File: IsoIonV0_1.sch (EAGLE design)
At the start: 52 parts, among them IC1 MCP3221, IC2 MCP4017-100K, IC4 TL072, IC5 TPS60400DBV

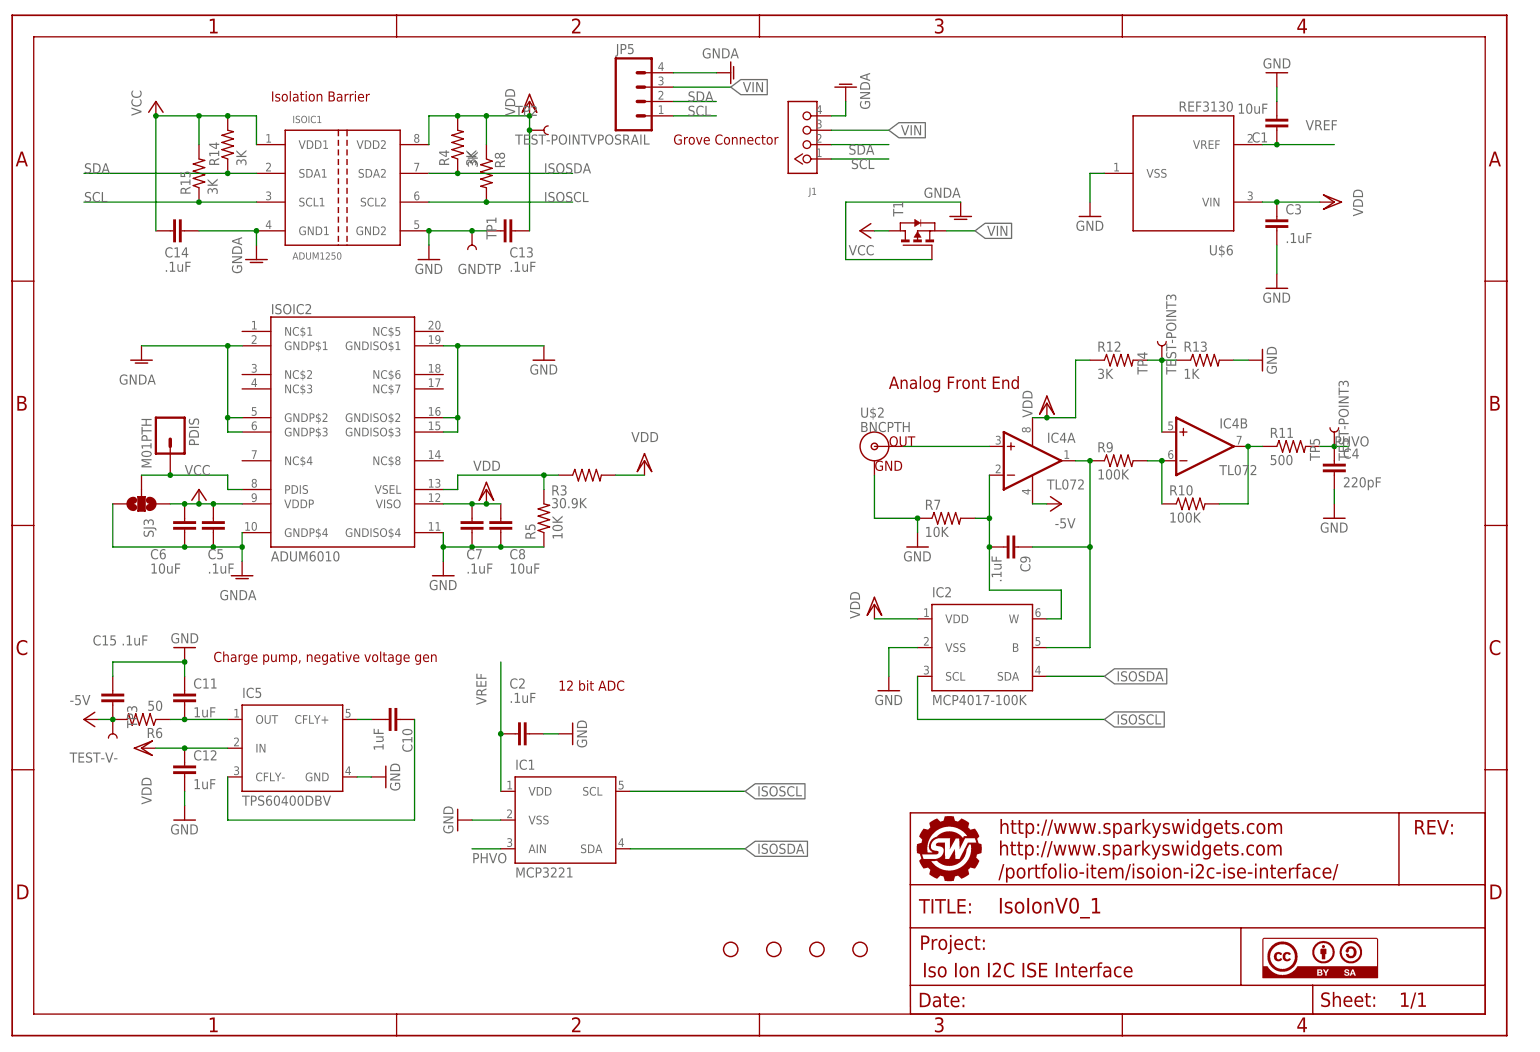
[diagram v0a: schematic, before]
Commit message: Cleaned up sch small silkscreen adjustment on brd
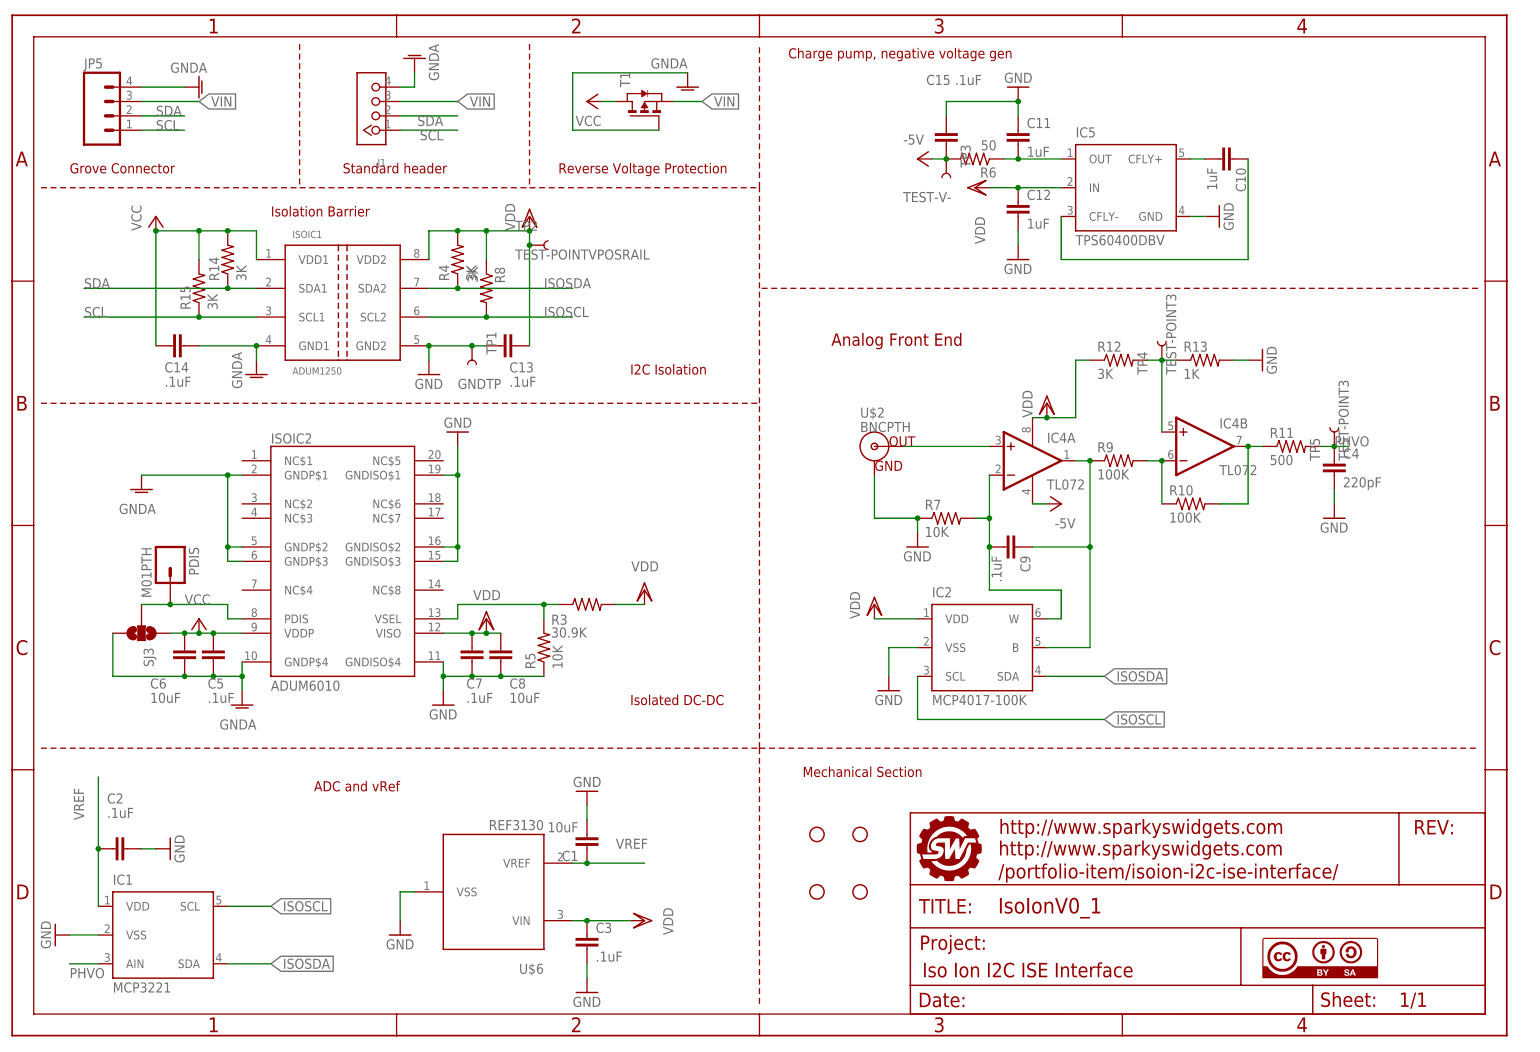
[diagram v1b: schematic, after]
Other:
- note added: "ADC and vRef"
- note added: "I2C Isolation"
- note added: "Isolated DC-DC"
- note added: "Mechanical Section"
- note added: "Reverse Voltage Protection"
- note added: "Standard header"
- note removed: "12 bit ADC"
- moved on the sheet: C1, C10, C11, C12, C13, C14, C15, C2, C3, C5, C6, C7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
